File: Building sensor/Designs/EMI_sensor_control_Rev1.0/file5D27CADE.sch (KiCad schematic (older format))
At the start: 37 parts

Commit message: Weekly Push
Weekly Push
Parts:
- removed C? (x2): C 10u, symbol Device:C
- removed C?: C 100u, symbol Device:C
- removed C?: C 2.2u, symbol Device:C
- removed CR?: B0540W-7-F, SOD123, symbol 2019-07-16_15-03-54:B0540W-7-F
- removed J?: Conn_01x03_Male, symbol Connector:Conn_01x03_Male
- removed L?: L 6.8u, symbol Device:L
- removed R?: R 22.1k, symbol Device:R
- removed R?: R 4.42k, symbol Device:R
- removed U?: LMR23610ADDAR, DDA8, symbol 2019-07-25_16-42-24:LMR23610ADDAR
- removed U?: ADR434ARZ, R_8, symbol 2019-07-22_20-43-49:ADR434ARZ
- added C10: C 10u, Capacitor_SMD:C_1210_3225Metric_Pad1.42x2.65mm_HandSolder, symbol Device:C
- added C12: C 2.2u, Capacitor_SMD:C_0603_1608Metric_Pad1.05x0.95mm_HandSolder, symbol Device:C
- added C14: C 100n, Capacitor_SMD:C_0603_1608Metric_Pad1.05x0.95mm_HandSolder, symbol Device:C
- added C16: C 330u, Capacitor_SMD:CP_Elec_5x5.3, symbol Device:C
- added C87: C 1.8n, Capacitor_SMD:C_0805_2012Metric_Pad1.15x1.40mm_HandSolder, symbol Device:C
- added D2: B340A-13-F, digikey-footprints:DO-214AC, symbol dk_Diodes-Rectifiers-Single:B340A-13-F
- added L1: L 6.8u, symbol Device:L
- added R15: R 4.42k, symbol Device:R
- added R16: R 22.1k, symbol Device:R
- added SW1: SW_SP3T, symbol Switch:SW_SP3T
- added U5: REF2041AIDDCT, symbol 2019-07-29_16-20-46:REF2041AIDDCT
- added U6: LMR23610ADDAR, symbol 2019-07-25_16-42-24:LMR23610ADDAR
- C1, C2, C3, C4, C9: renamed from C?; footprint (none) -> Capacitor_SMD:C_1210_3225Metric_Pad1.42x2.65mm_HandSolder
- C11: renamed from C?; value C 10u -> C 100n; footprint (none) -> Capacitor_SMD:C_0603_1608Metric_Pad1.05x0.95mm_HandSolder
- C13: renamed from C?; value C 0.1uf -> C 100n; footprint (none) -> Capacitor_SMD:C_0603_1608Metric_Pad1.05x0.95mm_HandSolder
- C15: renamed from C?; value C 0.1u -> C 100n; footprint (none) -> Capacitor_SMD:C_0603_1608Metric_Pad1.05x0.95mm_HandSolder
- C5: renamed from C?; footprint (none) -> Capacitor_SMD:C_0805_2012Metric_Pad1.15x1.40mm_HandSolder
- C6, C7: renamed from C?; footprint (none) -> Capacitor_SMD:C_1206_3216Metric_Pad1.42x1.75mm_HandSolder
- C8: renamed from C?; value C 33u -> C 68u; footprint (none) -> Capacitor_SMD:C_1206_3216Metric_Pad1.42x1.75mm_HandSolder
- gave numbers to parts that had none: 13
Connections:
- net labels added: Vref2.1, Vref4.1
- net labels removed: Vref
- wire segments 169 -> 179
- no-connect marks 6 -> 5
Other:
- moved on the sheet: BT1, C1, C11, C13, C15, C2, C3, C4, C5, C6, C7, C8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

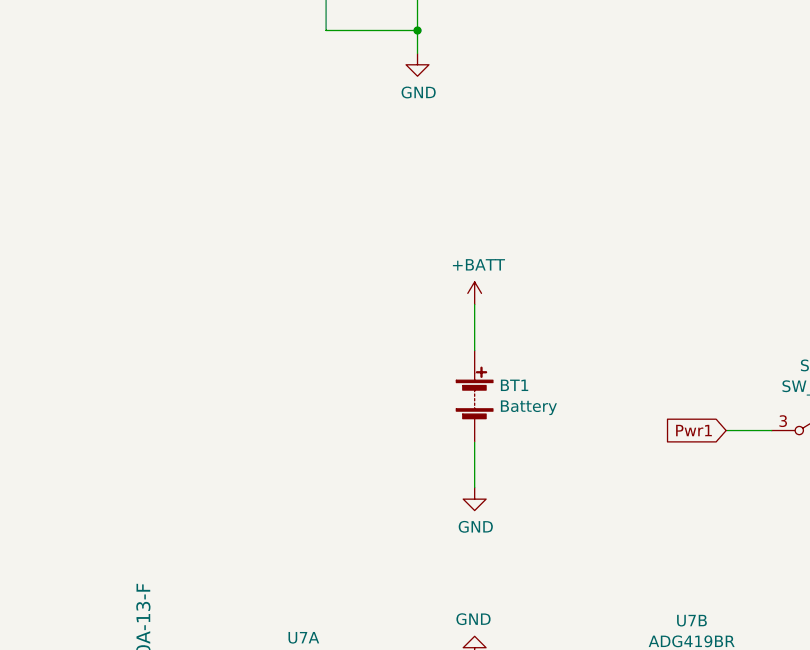
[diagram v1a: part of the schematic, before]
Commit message: Weekly Commit
Weekly Commit 08/09/2019
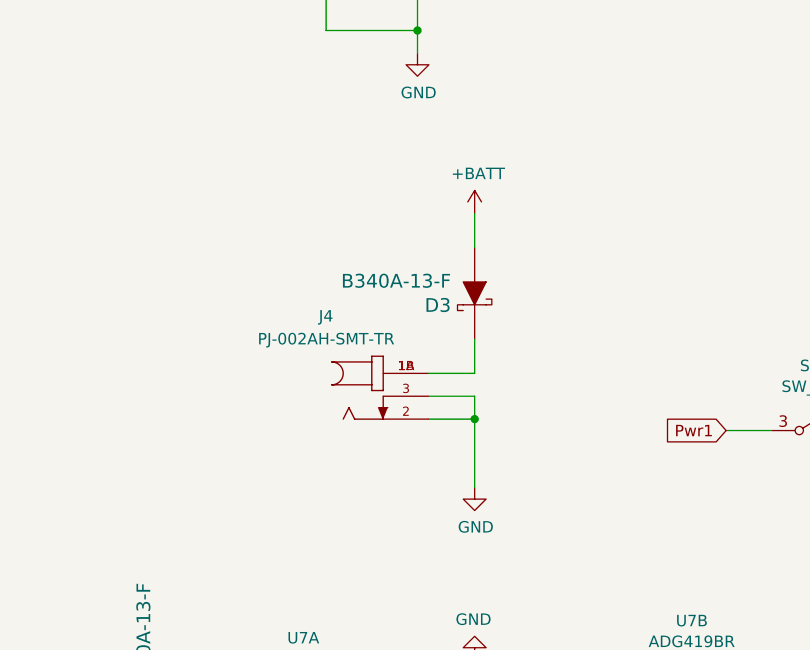
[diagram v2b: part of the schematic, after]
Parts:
- removed BT1: Battery, symbol Device:Battery
- added D3: B340A-13-F, digikey-footprints:DO-214AC, symbol dk_Diodes-Rectifiers-Single:B340A-13-F
- added J4: PJ-002AH-SMT-TR, PJ-002AH-SMT-TR:CUI_PJ-002AH-SMT-TR, symbol PJ-002AH-SMT-TR:PJ-002AH-SMT-TR
- L1: footprint (none) -> footprints:SRN6045-6R8Y
- R10, R11, R12, R13, R14, R9: footprint (none) -> Resistor_SMD:R_0805_2012Metric_Pad1.15x1.40mm_HandSolder
- R15, R16: footprint (none) -> Resistor_SMD:R_1206_3216Metric_Pad1.42x1.75mm_HandSolder
- SW1: footprint (none) -> Button_Switch_SMD:SW_SP3T_PCM13
- U5: footprint (none) -> footprints:REF2041AIDDCT
- U6: footprint (none) -> footprints:LMR23610ADDAR
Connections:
- net +BATT: now also D3.A
- net GND: now also J4.2, J4.3
- new net: D3.K, J4.1A (1), J4.1B (1)
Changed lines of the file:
@@
 F 0 "R11" V 6150 2100 50  0000 L CNN
 F 1 "R 120k" H 6220 2105 50  0000 L CNN
-F 2 "" V 6080 2150 50  0001 C CNN
+F 2 "Resistor_SMD:R_0805_2012Metric_Pad1.15x1.40mm_HandSolder" V 6080 2150 50  0001 C CNN
 F 3 "~" H 6150 2150 50  0001 C CNN
 	1    6150 2150
@@
 F 0 "R12" V 6150 2550 50  0000 L CNN
 F 1 "R 52.3k" H 6220 2555 50  0000 L CNN
-F 2 "" V 6080 2600 50  0001 C CNN
+F 2 "Resistor_SMD:R_0805_2012Metric_Pad1.15x1.40mm_HandSolder" V 6080 2600 50  0001 C CNN
 F 3 "~" H 6150 2600 50  0001 C CNN
 	1    6150 2600
@@
 	14900 8400 14900 8250
 $Comp
-L Device:Battery BT1
-U 1 1 5D2CA3E0
-P 13300 7100
-F 0 "BT1" H 13408 7146 50  0000 L CNN
-F 1 "Battery" H 13408 7055 50  0000 L CNN
-F 2 "" V 13300 7160 50  0001 C CNN
-F 3 "~" V 13300 7160 50  0001 C CNN
-	1    13300 7100
-	1    0    0    -1
-$EndComp
-$Comp
 L power:GND #PWR036
 U 1 1 5D2CBED6
@@
 L power:+BATT #PWR035
 U 1 1 5D2D6E3A
-P 13300 6700
-F 0 "#PWR035" H 13300 6550 50  0001 C CNN
-F 1 "+BATT" H 13315 6873 50  0000 C CNN
-F 2 "" H 13300 6700 50  0001 C CNN
-F 3 "" H 13300 6700 50  0001 C CNN
-	1    13300 6700
+P 13300 6300
+F 0 "#PWR035" H 13300 6150 50  0001 C CNN
+F 1 "+BATT" H 13315 6473 50  0000 C CNN
+F 2 "" H 13300 6300 50  0001 C CNN
+F 3 "" H 13300 6300 50  0001 C CNN
+	1    13300 6300
 	1    0    0    -1
 $EndComp
@@
 F 0 "R13" V 6150 9200 50  0000 L CNN
 F 1 "R 38.3k" H 6220 9205 50  0000 L CNN
-F 2 "" V 6080 9250 50  0001 C CNN
+F 2 "Resistor_SMD:R_0805_2012Metric_Pad1.15x1.40mm_HandSolder" V 6080 9250 50  0001 C CNN
 F 3 "~" H 6150 9250 50  0001 C CNN
 	1    6150 9250
@@
 F 0 "R14" V 6150 9650 50  0000 L CNN
 F 1 "R 25.5k" H 6220 9655 50  0000 L CNN
-F 2 "" V 6080 9700 50  0001 C CNN
+F 2 "Resistor_SMD:R_0805_2012Metric_Pad1.15x1.40mm_HandSolder" V 6080 9700 50  0001 C CNN
 F 3 "~" H 6150 9700 50  0001 C CNN
 	1    6150 9700
@@
 F 0 "R9" V 4950 6500 50  0000 L CNN
 F 1 "R 102k" H 5020 6505 50  0000 L CNN
-F 2 "" V 4880 6550 50  0001 C CNN
+F 2 "Resistor_SMD:R_0805_2012Metric_Pad1.15x1.40mm_HandSolder" V 4880 6550 50  0001 C CNN
 F 3 "~" H 4950 6550 50  0001 C CNN
 	1    4950 6550
@@
 F 0 "R10" V 4950 6900 50  0000 L CNN
 F 1 "R 25.5k" H 5020 6905 50  0000 L CNN
-F 2 "" V 4880 6950 50  0001 C CNN
+F 2 "Resistor_SMD:R_0805_2012Metric_Pad1.15x1.40mm_HandSolder" V 4880 6950 50  0001 C CNN
 F 3 "~" H 4950 6950 50  0001 C CNN
 	1    4950 6950
@@
 F 0 "U5" H 11500 5287 60  0000 C CNN
 F 1 "REF2041AIDDCT" H 11500 5181 60  0000 C CNN
-F 2 "" H 11500 5140 60  0001 C CNN
+F 2 "footprints:REF2041AIDDCT" H 11500 5140 60  0001 C CNN
 F 3 "" H 10700 4900 60  0000 C CNN
 	1    10700 4900
@@
 F 0 "R15" V 13700 2750 50  0000 L CNN
 F 1 "R 4.42k" H 13770 2755 50  0000 L CNN
-F 2 "" V 13630 2800 50  0001 C CNN
+F 2 "Resistor_SMD:R_1206_3216Metric_Pad1.42x1.75mm_HandSolder" V 13630 2800 50  0001 C CNN
 F 3 "~" H 13700 2800 50  0001 C CNN
 	1    13700 2800
@@
 F 0 "L1" V 13119 2500 50  0000 C CNN
 F 1 "L 6.8u" V 13210 2500 50  0000 C CNN
-F 2 "" H 13300 2500 50  0001 C CNN
+F 2 "footprints:SRN6045-6R8Y" H 13300 2500 50  0001 C CNN
 F 3 "~" H 13300 2500 50  0001 C CNN
 	1    13300 2500
@@
 F 0 "R16" V 13700 3250 50  0000 L CNN
 F 1 "R 22.1k" H 13770 3255 50  0000 L CNN
-F 2 "" V 13630 3300 50  0001 C CNN
+F 2 "Resistor_SMD:R_1206_3216Metric_Pad1.42x1.75mm_HandSolder" V 13630 3300 50  0001 C CNN
 F 3 "~" H 13700 3300 50  0001 C CNN
 	1    13700 3300
@@
 F 0 "U6" H 13200 2787 60  0000 C CNN
 F 1 "LMR23610ADDAR" H 13200 2681 60  0000 C CNN
-F 2 "" H 13200 2640 60  0001 C CNN
+F 2 "footprints:LMR23610ADDAR" H 13200 2640 60  0001 C CNN
 F 3 "" H 12300 2400 60  0000 C CNN
 	1    12300 2400
@@
 	13450 5000 12650 5000
 Connection ~ 12650 5000
-Wire Wire Line
-	13300 7500 13300 7300
-Wire Wire Line
-	13300 6900 13300 6700
 $Comp
 L Switch:SW_SP3T SW1
@@
 F 0 "SW1" H 14800 7533 50  0000 C CNN
 F 1 "SW_SP3T" H 14800 7442 50  0000 C CNN
-F 2 "" H 14175 7425 50  0001 C CNN
+F 2 "Button_Switch_SMD:SW_SP3T_PCM13" H 14175 7425 50  0001 C CNN
 F 3 "~" H 14175 7425 50  0001 C CNN
 	1    14800 7250
@@
 Wire Wire Line
 	13700 2600 13700 2650
+$Comp
+L PJ-002AH-SMT-TR:PJ-002AH-SMT-TR J4
+U 1 1 5D4ED109
+P 12900 7100
+F 0 "J4" H 12650 7450 50  0000 C CNN
+F 1 "PJ-002AH-SMT-TR" H 12650 7350 50  0000 C CNN
+F 2 "PJ-002AH-SMT-TR:CUI_PJ-002AH-SMT-TR" H 12900 7100 50  0001 L BNN
+F 3 "" H 12900 7100 50  0001 L BNN
+F 4 "PJ-002AH-SMT-TR" H 12900 7100 50  0001 L BNN "Field4"
+F 5 "https://www.cui.com/product/interconnect/connectors/dc-power-connectors/jacks/pj-002ah-smt-tr?utm_source=snapeda.com&utm_medium=referral&utm_campaign=snapedaBOM" H 12900 7100 50  0001 L BNN "Field5"
+F 6 "https://www.digikey.com/product-detail/en/cui-inc/PJ-002AH-SMT-TR/CP-002AHPJCT-ND/669692?utm_source=snapeda&utm_medium=aggregator&utm_campaign=symbol" H 12900 7100 50  0001 L BNN "Field6"
+F 7 "2.0 x 6.5 mm, 5.0 A, Horizontal, Surface Mount _SMT_, Dc Power Jack Connector" H 12900 7100 50  0001 L BNN "Field7"
+F 8 "CP-002AHPJCT-ND" H 12900 7100 50  0001 L BNN "Field8"
+F 9 "None" H 12900 7100 50  0001 L BNN "Field9"
+	1    12900 7100
+	1    0    0    -1
+$EndComp
+Wire Wire Line
+	13300 7000 13100 7000
+Wire Wire Line
+	13100 7100 13300 7100
+Wire Wire Line
+	13300 7100 13300 7200
+Wire Wire Line
+	13100 7200 13300 7200
+Connection ~ 13300 7200
+Wire Wire Line
+	13300 7200 13300 7500
+$Comp
+L dk_Diodes-Rectifiers-Single:B340A-13-F D3
+U 1 1 5D50F1A3
+P 13300 6650
+F 0 "D3" V 13353 6547 60  0000 R CNN
+F 1 "B340A-13-F" V 13247 6547 60  0000 R CNN
+F 2 "digikey-footprints:DO-214AC" H 13500 6850 60  0001 L CNN
+F 3 "https://www.diodes.com/assets/Datasheets/ds30891.pdf" H 13500 6950 60  0001 L CNN
+F 4 "B340A-FDICT-ND" H 13500 7050 60  0001 L CNN "Digi-Key_PN"
+F 5 "B340A-13-F" H 13500 7150 60  0001 L CNN "MPN"
+F 6 "Discrete Semiconductor Products" H 13500 7250 60  0001 L CNN "Category"
+F 7 "Diodes - Rectifiers - Single" H 13500 7350 60  0001 L CNN "Family"
+F 8 "https://www.diodes.com/assets/Datasheets/ds30891.pdf" H 13500 7450 60  0001 L CNN "DK_Datasheet_Link"
+F 9 "/product-detail/en/diodes-incorporated/B340A-13-F/B340A-FDICT-ND/725054" H 13500 7550 60  0001 L CNN "DK_Detail_Page"
+F 10 "DIODE SCHOTTKY 40V 3A SMA" H 13500 7650 60  0001 L CNN "Description"
+F 11 "Diodes Incorporated" H 13500 7750 60  0001 L CNN "Manufacturer"
+F 12 "Active" H 13500 7850 60  0001 L CNN "Status"
+	1    13300 6650
+	0    1    1    0
+$EndComp
+Wire Wire Line
+	13300 6300 13300 6450
+Wire Wire Line
+	13300 6850 13300 7000
 $EndSCHEMATC
